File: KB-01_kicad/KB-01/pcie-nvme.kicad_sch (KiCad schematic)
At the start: 20 parts, among them J1 Bus_M.2_Socket_M, M1 M.2 Solder Nut, M2 M.2 Screw, U4 ASEK-32.768KHZ-L-R-T, U5 AP3441SHE-7B

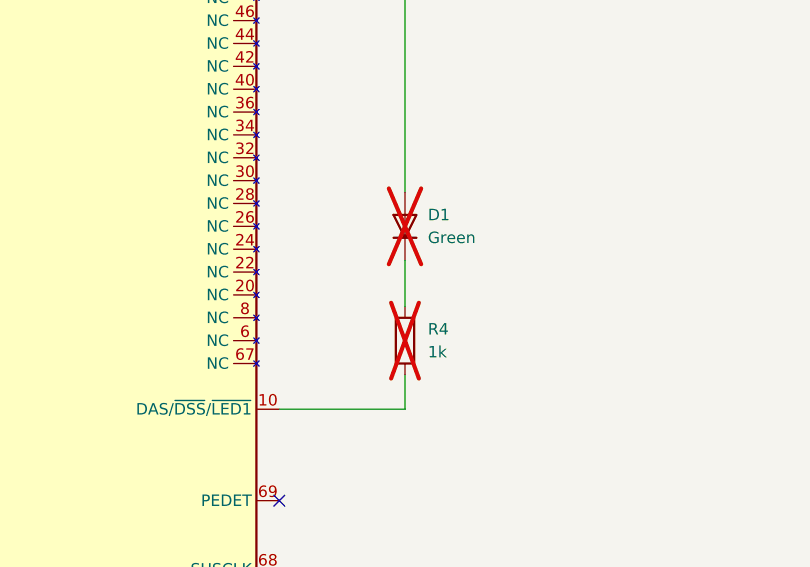
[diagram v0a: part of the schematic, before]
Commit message: everything
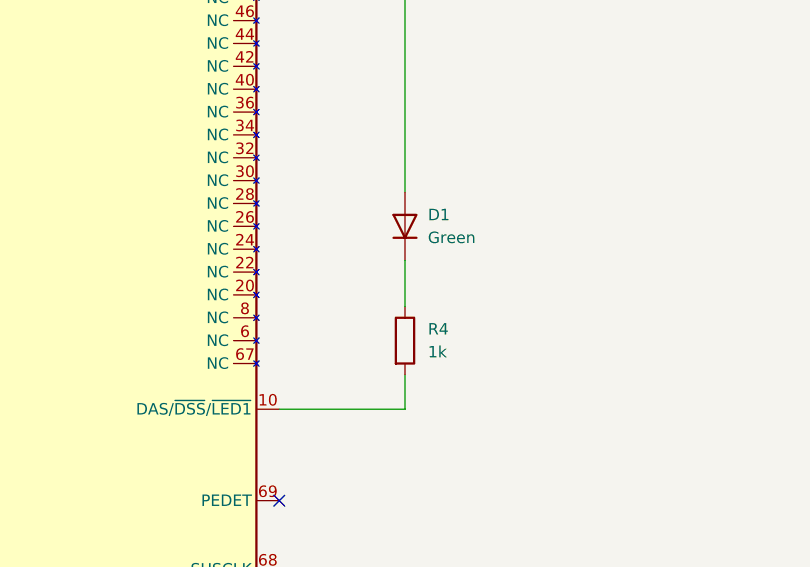
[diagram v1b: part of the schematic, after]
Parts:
- D1, R4: now fitted; now in the parts list
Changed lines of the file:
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@@
 		(unit 1)
 		(exclude_from_sim no)
-		(in_bom no)
-		(on_board yes)
-		(dnp yes)
+		(in_bom yes)
+		(on_board yes)
+		(dnp no)
 		(fields_autoplaced yes)
 		(property "Reference" "R4"
@@
 		(unit 1)
 		(exclude_from_sim no)
-		(in_bom no)
-		(on_board yes)
-		(dnp yes)
+		(in_bom yes)
+		(on_board yes)
+		(dnp no)
 		(fields_autoplaced yes)
 		(property "Reference" "D1"

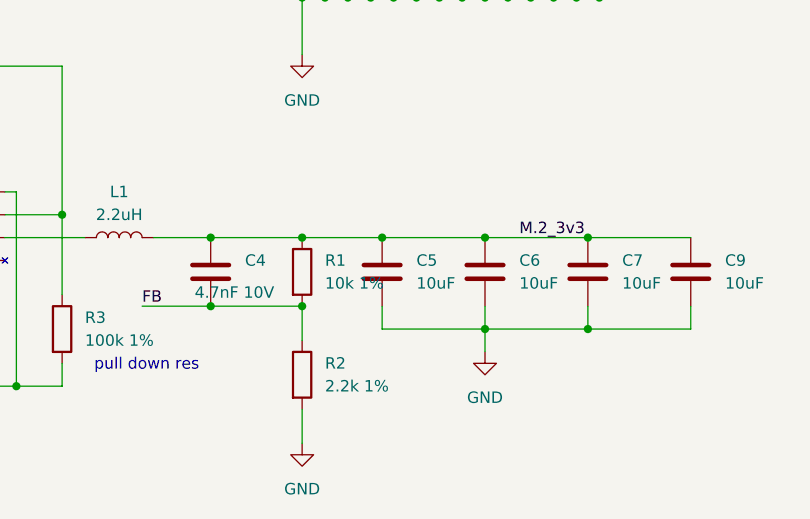
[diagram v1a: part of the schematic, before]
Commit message: all
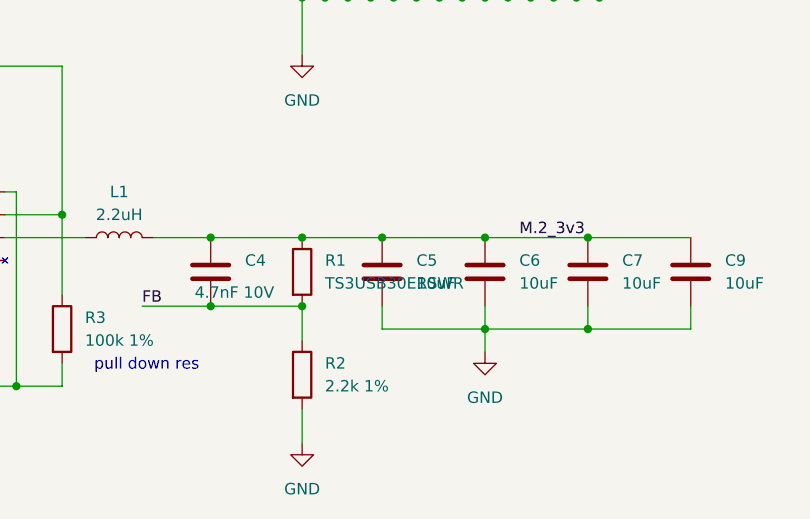
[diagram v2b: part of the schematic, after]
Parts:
- R1: value 10k 1% -> TS3USB30ERSWR; footprint Resistor_SMD:R_0603_1608Metric_Pad0.98x0.95mm_HandSolder -> Package_DFN_QFN:UQFN-10_1.4x1.8mm_P0.4mm; mouser 603-RT0603FRE1310KL -> 595-TS3USB30ERSWR

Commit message: all
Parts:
- D1: mouser (none) -> 859-LTST-C190KGKT
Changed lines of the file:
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@@
+			)
+		)
+		(property "mouser" "859-LTST-C190KGKT"
+			(at 189.23 81.28 90)
+			(hide yes)
+			(show_name no)
+			(do_not_autoplace no)
+			(effects
+				(font
+					(size 1.27 1.27)
+				)
 			)
 		)

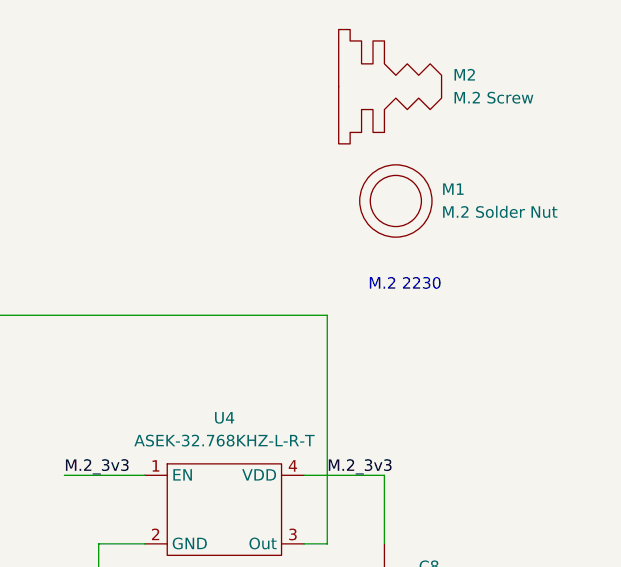
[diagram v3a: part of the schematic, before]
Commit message: all
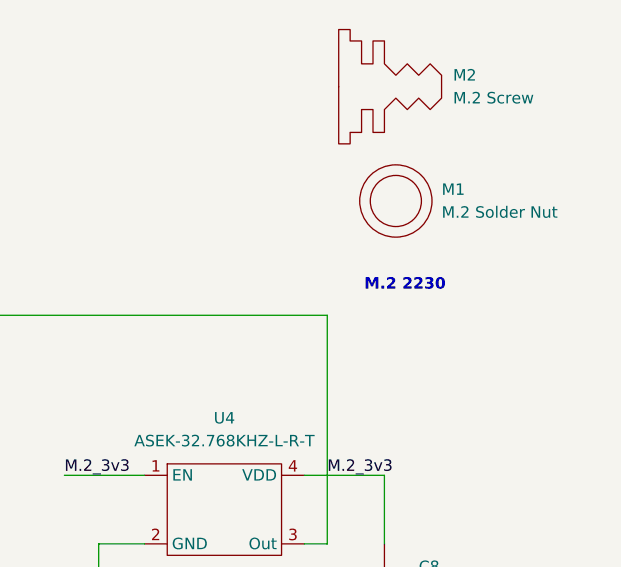
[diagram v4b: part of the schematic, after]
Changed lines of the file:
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@@
 			(font
 				(size 1.27 1.27)
+				(thickness 0.254)
+				(bold yes)
 			)
 		)

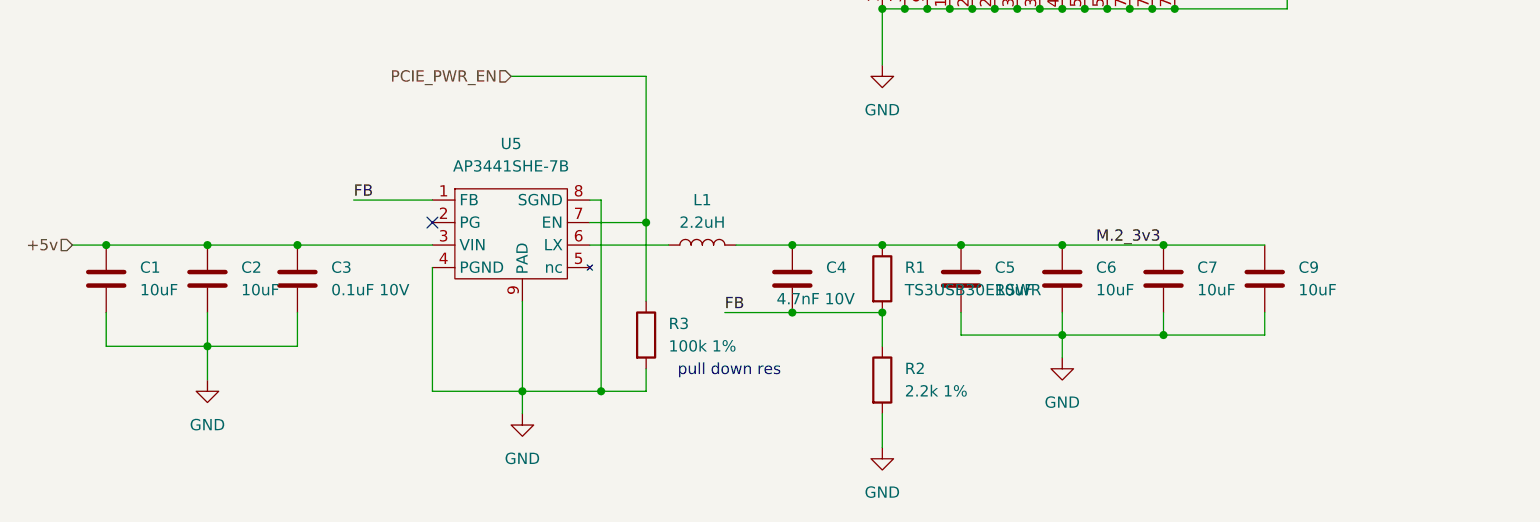
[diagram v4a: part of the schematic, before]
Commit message: all
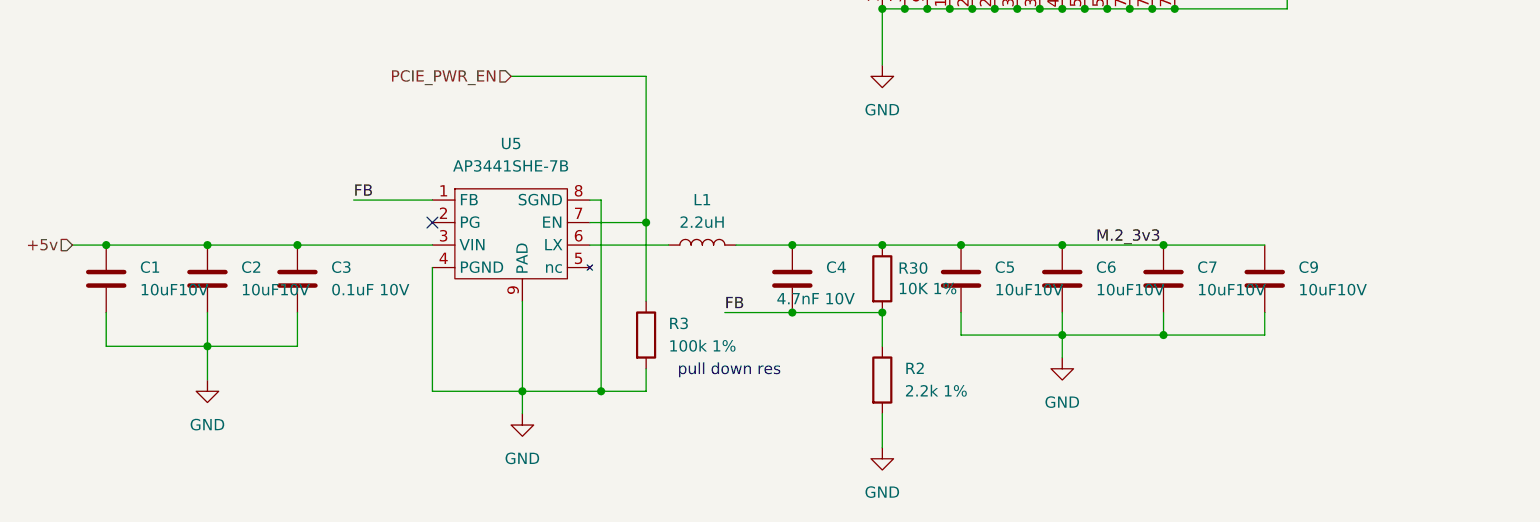
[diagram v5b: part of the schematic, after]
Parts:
- removed R1: TS3USB30ERSWR, Package_DFN_QFN:UQFN-10_1.4x1.8mm_P0.4mm, symbol Device:R
- added R30: 10K 1%, Resistor_SMD:R_0603_1608Metric_Pad0.98x0.95mm_HandSolder, symbol Device:R
- C1, C2, C5, C6, C7, C9: value 10uF -> 10uF10V
- L1: mouser (none) -> 652-SRP5030CC-2R2M
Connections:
- net FB: now also R30.2
- net M.2_3v3: now also R30.1
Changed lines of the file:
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@@
 	)
 	(junction
+		(at 129.54 173.99)
+		(diameter 0)
+		(color 0 0 0 0)
+	)
+	(junction
 		(at 97.79 182.88)
 		(diameter 0)
@@
 	)
 	(junction
-		(at 129.54 166.37)
+		(at 213.36 152.4)
 		(diameter 0)
 		(color 0 0 0 0)
 	)
 	(junction
-		(at 213.36 152.4)
+		(at 138.43 166.37)
 		(diameter 0)
 		(color 0 0 0 0)
 	)
 	(junction
-		(at 138.43 166.37)
+		(at 129.54 166.37)
 		(diameter 0)
 		(color 0 0 0 0)
@@
 	)
 	(junction
-		(at 129.54 173.99)
-		(diameter 0)
-		(color 0 0 0 0)
-	)
-	(junction
 		(at 162.56 139.7)
 		(diameter 0)
@@
 	(wire
 		(pts
-			(xy 129.54 166.37) (xy 138.43 166.37)
+			(xy 119.38 166.37) (xy 129.54 166.37)
 		)
 		(stroke
@@
 	(wire
 		(pts
-			(xy 119.38 166.37) (xy 129.54 166.37)
-		)
-		(stroke
-			(width 0)
-			(type default)
-		)
-	)
-	(wire
-		(pts
 			(xy 154.94 139.7) (xy 157.48 139.7)
 		)
@@
 	(wire
 		(pts
+			(xy 129.54 166.37) (xy 138.43 166.37)
+		)
+		(stroke
+			(width 0)
+			(type default)
+		)
+	)
+	(wire
+		(pts
 			(xy 53.34 177.8) (xy 53.34 181.61)
 		)
@@
 			)
 		)
-		(property "Value" "10uF"
+		(property "Value" "10uF10V"
 			(at 176.53 171.4499 0)
 			(show_name no)
@@
 			)
 		)
-		(property "Value" "10uF"
+		(property "Value" "10uF10V"
 			(at 57.15 171.4499 0)
 			(show_name no)
@@
 	)
 	(symbol
-		(lib_id "Device:R")
-		(at 129.54 170.18 0)
-		(unit 1)
-		(body_style 1)
-		(exclude_from_sim no)
-		(in_bom yes)
-		(on_board yes)
-		(in_pos_files yes)
-		(dnp no)
-		(fields_autoplaced yes)
-		(property "Reference" "R1"
-			(at 132.08 168.9099 0)
-			(show_name no)
-			(do_not_autoplace no)
-			(effects
-				(font
-					(size 1.27 1.27)
-				)
-				(justify left)
-			)
-		)
-		(property "Value" "TS3USB30ERSWR"
-			(at 132.08 171.4499 0)
-			(show_name no)
-			(do_not_autoplace no)
-			(effects
-				(font
-					(size 1.27 1.27)
-				)
-				(justify left)
-			)
-		)
-		(property "Footprint" "Package_DFN_QFN:UQFN-10_1.4x1.8mm_P0.4mm"
-			(at 127.762 170.18 90)
-			(hide yes)
-			(show_name no)
-			(do_not_autoplace no)
-			(effects
-				(font
-					(size 1.27 1.27)
-				)
-			)
-		)
-		(property "Datasheet" "https://www.ti.com/lit/ds/symlink/ts3usb30e.pdf"
-			(at 129.54 170.18 0)
-			(hide yes)
-			(show_name no)
-			(do_not_autoplace no)
-			(effects
-				(font
-					(size 1.27 1.27)
-				)
-			)
-		)
-		(property "Description" "ESD-Protected, High-Speed USB 2.0 (480-Mbps) 1:2 Multiplexer/Demultiplexer Switch With Single Enable, UQFN-10"
-			(at 129.54 170.18 0)
-			(hide yes)
-			(show_name no)
-			(do_not_autoplace no)
-			(effects
-				(font
-					(size 1.27 1.27)
-				)
-			)
-		)
-		(property "mouser" "595-TS3USB30ERSWR"
-			(at 129.54 170.18 0)
-			(hide yes)
-			(show_name no)
-			(do_not_autoplace no)
-			(effects
-				(font
-					(size 1.27 1.27)
-				)
-			)
-		)
-		(pin "1"
-		)
-		(pin "2"
-		)
-		(instances
-			(project "KB-01"
-				(path "/e6144e29-1dc4-45a8-93e7-988a20131b94/e474c326-f80b-4652-be93-3ce49aa7493e"
-					(reference "R1")
-					(unit 1)
-				)
-			)
-		)
-	)
-	(symbol
 		(lib_id "Device:C")
 		(at 245.11 148.59 0)
@@
 			)
 		)
-		(property "Value" "10uF"
+		(property "Value" "10uF10V"
 			(at 165.1 171.4499 0)
 			(show_name no)
@@
 			)
 		)
-		(property "Value" "10uF"
+		(property "Value" "10uF10V"
 			(at 45.72 171.4499 0)
 			(show_name no)
@@
 	)
 	(symbol
+		(lib_id "Device:R")
+		(at 129.54 170.18 0)
+		(unit 1)
+		(body_style 1)
+		(exclude_from_sim no)
+		(in_bom yes)
+		(on_board yes)
+		(in_pos_files yes)
+		(dnp no)
+		(property "Reference" "R30"
+			(at 131.318 169.0116 0)
+			(show_name no)
+			(do_not_autoplace no)
+			(effects
+				(font
+					(size 1.27 1.27)
+				)
+				(justify left)
+			)
+		)
+		(property "Value" "10K 1%"
+			(at 131.318 171.323 0)
+			(show_name no)
+			(do_not_autoplace no)
+			(effects
+				(font
+					(size 1.27 1.27)
+				)
+				(justify left)
+			)
+		)
+		(property "Footprint" "Resistor_SMD:R_0603_1608Metric_Pad0.98x0.95mm_HandSolder"
+			(at 127.762 170.18 90)
+			(hide yes)
+			(show_name no)
+			(do_not_autoplace no)
+			(effects
+				(font
+					(size 1.27 1.27)
+				)
+			)
+		)
+		(property "Datasheet" "https://fscdn.rohm.com/en/products/databook/datasheet/passive/resistor/chip_resistor/mcr-e.pdf"
+			(at 129.54 170.18 0)
+			(hide yes)
+			(show_name no)
+			(do_not_autoplace no)
+			(effects
+				(font
+					(size 1.27 1.27)
+				)
+			)
+		)
+		(property "Description" ""
+			(at 129.54 170.18 0)
+			(hide yes)
+			(show_name no)
+			(do_not_autoplace no)
+			(effects
+				(font
+					(size 1.27 1.27)
+				)
+			)
+		)
+		(property "Field4" "Farnell"
+			(at 129.54 170.18 0)
+			(hide yes)
+			(show_name no)
+			(do_not_autoplace no)
+			(effects
+				(font
+					(size 1.27 1.27)
+				)
+			)
+		)
+		(property "Field5" ""
+			(at 129.54 170.18 0)
+			(hide yes)
+			(show_name no)
+			(do_not_autoplace no)
+			(effects
+				(font
+					(size 1.27 1.27)
+				)
+			)
+		)
+		(property "Field7" "Rohm"
+			(at 129.54 170.18 0)
+			(hide yes)
+			(show_name no)
+			(do_not_autoplace no)
+			(effects
+				(font
+					(size 1.27 1.27)
+				)
+			)
+		)
+		(property "Field6" "MCR01MZPF1002"
+			(at 129.54 170.18 0)
+			(hide yes)
+			(show_name no)
+			(do_not_autoplace no)
+			(effects
+				(font
+					(size 1.27 1.27)
+				)
+			)
+		)
+		(property "Part Description" "Resistor 10K M1005 1% 63mW"
+			(at 129.54 170.18 0)
+			(hide yes)
+			(show_name no)
+			(do_not_autoplace no)
+			(effects
+				(font
+					(size 1.27 1.27)
+				)
+			)
+		)
+		(property "mouser" "708-RMCF0603FT10K0"
+			(at 129.54 170.18 0)
+			(hide yes)
+			(show_name no)
+			(do_not_autoplace no)
+			(effects
+				(font
+					(size 1.27 1.27)
+				)
+			)
+		)
+		(pin "1"
+		)
+		(pin "2"
+		)
+		(instances
+			(project "KB-01"
+				(path "/e6144e29-1dc4-45a8-93e7-988a20131b94/e474c326-f80b-4652-be93-3ce49aa7493e"
+					(reference "R30")
+					(unit 1)
+				)
+			)
+		)
+	)
+	(symbol
 		(lib_id "power:GND")
 		(at 88.9 185.42 0)
@@
 			)
 		)
-		(property "Value" "10uF"
+		(property "Value" "10uF10V"
 			(at 142.24 171.4499 0)
 			(show_name no)
@@
 			)
 		)
-		(property "Value" "10uF"
+		(property "Value" "10uF10V"
 			(at 153.67 171.4499 0)
 			(show_name no)
@@
 			(hide yes)
 			(show_name no)
+			(do_not_autoplace no)
+			(effects
+				(font
+					(size 1.27 1.27)
+				)
+			)
+		)
+		(property "mouser" "652-SRP5030CC-2R2M"
+			(at 109.22 166.37 90)
+			(hide yes)
+			(show_name no)

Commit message: all
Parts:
- R4: mouser 594-MCT06030C2201FP5 -> 652-CR0603FX-1001ELF
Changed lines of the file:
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@@
 			)
 		)
-		(property "mouser" "594-MCT06030C2201FP5 "
+		(property "mouser" "652-CR0603FX-1001ELF "
 			(at 189.23 93.98 0)
 			(hide yes)
